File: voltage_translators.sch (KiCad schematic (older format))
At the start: 31 parts, among them IC201 GTL2003PW, IC202 GTL2003PW, IC203 GTL2003PW, IC204 GTL2003PW, IC205 GTL2003PW

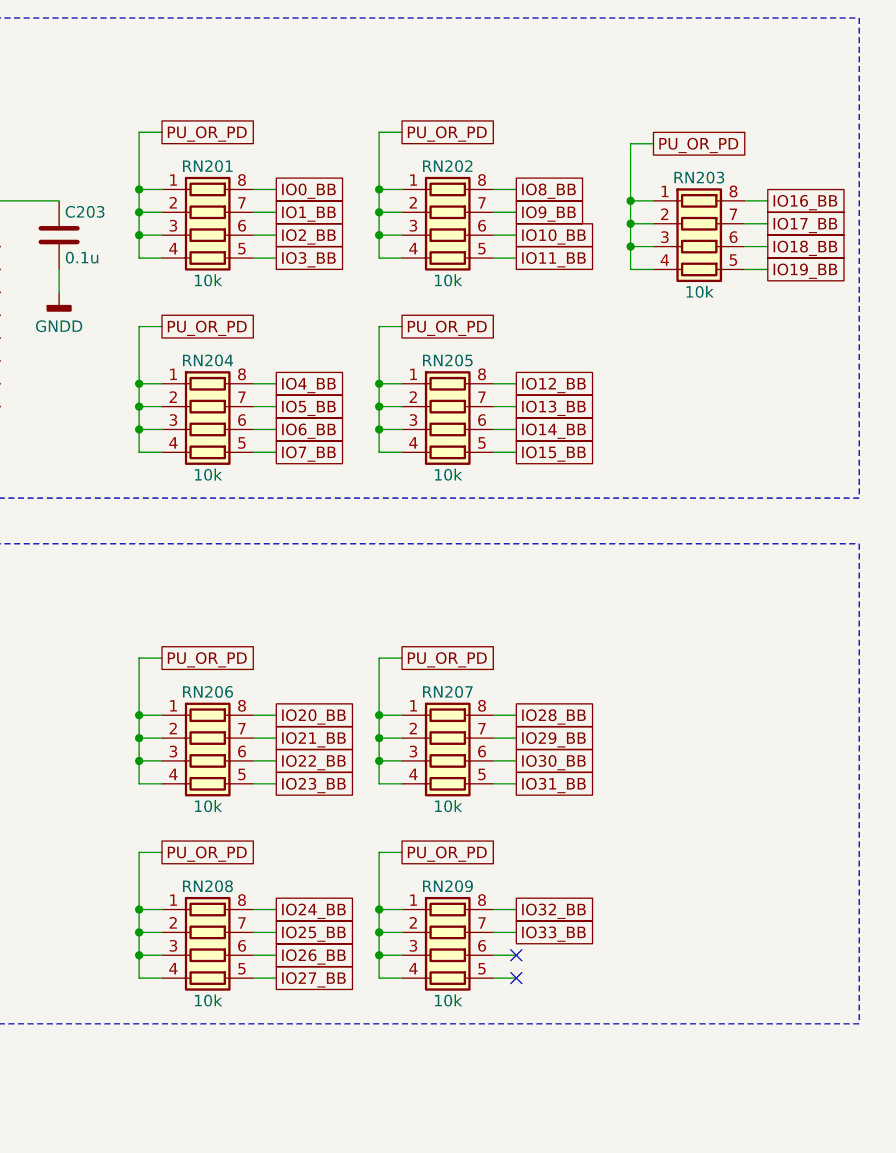
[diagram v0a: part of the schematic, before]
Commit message: revision 1.1 before via stitching
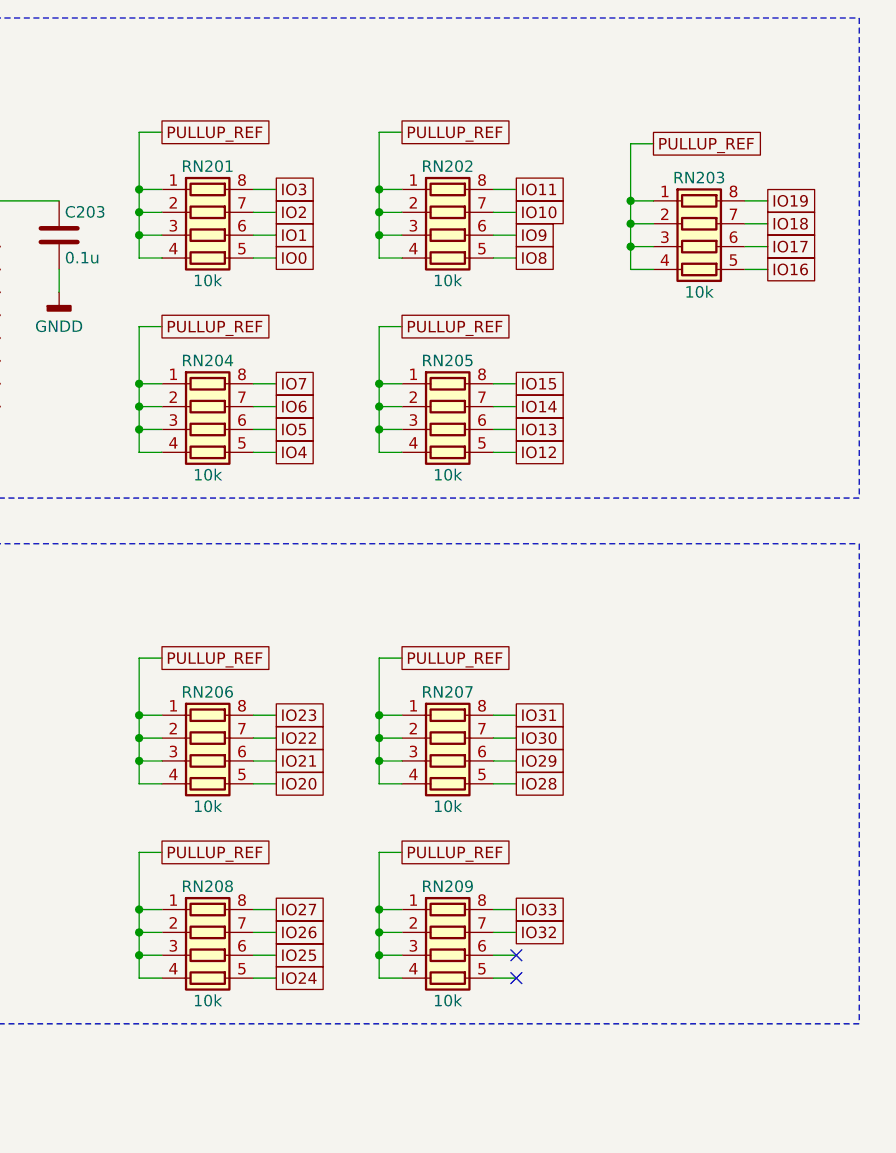
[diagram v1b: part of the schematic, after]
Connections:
- net IO0: now also RN201.5 (R4.2)
- net IO0_BB: no longer RN201.8 (R1.2)
- net IO1: now also RN201.6 (R3.2)
- net IO10: now also RN202.7 (R2.2)
- net IO10_BB: no longer RN202.6 (R3.2)
- net IO11: now also RN202.8 (R1.2)
- net IO11_BB: no longer RN202.5 (R4.2)
- net IO12: now also RN205.5 (R4.2)
- net IO12_BB: no longer RN205.8 (R1.2)
- net IO13: now also RN205.6 (R3.2)
- net IO13_BB: no longer RN205.7 (R2.2)
- net IO14: now also RN205.7 (R2.2)
- net IO14_BB: no longer RN205.6 (R3.2)
- net IO15: now also RN205.8 (R1.2)
- net IO15_BB: no longer RN205.5 (R4.2)
- net IO16: now also RN203.5 (R4.2)
- net IO16_BB: no longer RN203.8 (R1.2)
- net IO17: now also RN203.6 (R3.2)
- net IO17_BB: no longer RN203.7 (R2.2)
- net IO18: now also RN203.7 (R2.2)
- net IO18_BB: no longer RN203.6 (R3.2)
- net IO19: now also RN203.8 (R1.2)
- net IO19_BB: no longer RN203.5 (R4.2)
- net IO1_BB: no longer RN201.7 (R2.2)
- net IO2: now also RN201.7 (R2.2)
- net IO20: now also RN206.5 (R4.2)
- net IO20_BB: no longer RN206.8 (R1.2)
- net IO21: now also RN206.6 (R3.2)
- net IO21_BB: no longer RN206.7 (R2.2)
- net IO22: now also RN206.7 (R2.2)
- net IO22_BB: no longer RN206.6 (R3.2)
- net IO23: now also RN206.8 (R1.2)
- net IO23_BB: no longer RN206.5 (R4.2)
- net IO24: now also RN208.5 (R4.2)
- net IO24_BB: no longer RN208.8 (R1.2)
- net IO25: now also RN208.6 (R3.2)
- net IO25_BB: no longer RN208.7 (R2.2)
- net IO26: now also RN208.7 (R2.2)
- net IO26_BB: no longer RN208.6 (R3.2)
- net IO27: now also RN208.8 (R1.2)
- net IO27_BB: no longer RN208.5 (R4.2)
- net IO28: now also RN207.5 (R4.2)
- net IO28_BB: no longer RN207.8 (R1.2)
- net IO29: now also RN207.6 (R3.2)
- net IO29_BB: no longer RN207.7 (R2.2)
- net IO2_BB: no longer RN201.6 (R3.2)
- net IO3: now also RN201.8 (R1.2)
- net IO30: now also RN207.7 (R2.2)
- net IO30_BB: no longer RN207.6 (R3.2)
- net IO31: now also RN207.8 (R1.2)
- net IO31_BB: no longer RN207.5 (R4.2)
- net IO32: now also RN209.7 (R2.2)
- net IO32_BB: no longer RN209.8 (R1.2)
- net IO33: now also RN209.8 (R1.2)
- net IO33_BB: no longer RN209.7 (R2.2)
- net IO3_BB: no longer RN201.5 (R4.2)
- net IO4: now also RN204.5 (R4.2)
- net IO4_BB: no longer RN204.8 (R1.2)
- net IO5: now also RN204.6 (R3.2)
- net IO5_BB: no longer RN204.7 (R2.2)
- net IO6: now also RN204.7 (R2.2)
- net IO6_BB: no longer RN204.6 (R3.2)
- net IO7: now also RN204.8 (R1.2)
- net IO7_BB: no longer RN204.5 (R4.2)
- net IO8: now also RN202.5 (R4.2)
- net IO8_BB: no longer RN202.8 (R1.2)
- net IO9: now also RN202.6 (R3.2)
- net IO9_BB: no longer RN202.7 (R2.2)
- net PU_OR_PD renamed PULLUP_REF
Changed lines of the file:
@@
 encoding utf-8
 Sheet 2 2
-Title ""
+Title "BeagleBone Parallel Port Cape"
 Date ""
-Rev ""
-Comp ""
+Rev "1.1"
+Comp "Machine Koder"
 Comment1 ""
 Comment2 ""
@@
 	0    1    1    0
 $EndComp
+Text GLabel 8550 1750 2    50   UnSpc ~ 0
+IO0
+Text GLabel 8550 1650 2    50   UnSpc ~ 0
+IO1
+Text GLabel 8550 1550 2    50   UnSpc ~ 0
+IO2
 Text GLabel 8550 1450 2    50   UnSpc ~ 0
-IO0_BB
-Text GLabel 8550 1550 2    50   UnSpc ~ 0
-IO1_BB
-Text GLabel 8550 1650 2    50   UnSpc ~ 0
-IO2_BB
-Text GLabel 8550 1750 2    50   UnSpc ~ 0
-IO3_BB
+IO3
 $Comp
 L R_Pack04 RN204
@@
 	0    1    1    0
 $EndComp
+Text GLabel 8550 2600 2    50   UnSpc ~ 0
+IO4
+Text GLabel 8550 2500 2    50   UnSpc ~ 0
+IO5
+Text GLabel 8550 2400 2    50   UnSpc ~ 0
+IO6
 Text GLabel 8550 2300 2    50   UnSpc ~ 0
-IO4_BB
-Text GLabel 8550 2400 2    50   UnSpc ~ 0
-IO5_BB
-Text GLabel 8550 2500 2    50   UnSpc ~ 0
-IO6_BB
-Text GLabel 8550 2600 2    50   UnSpc ~ 0
-IO7_BB
+IO7
 $Comp
 L R_Pack04 RN202
@@
 	0    1    1    0
 $EndComp
+Text GLabel 9600 1750 2    50   UnSpc ~ 0
+IO8
+Text GLabel 9600 1650 2    50   UnSpc ~ 0
+IO9
+Text GLabel 9600 1550 2    50   UnSpc ~ 0
+IO10
 Text GLabel 9600 1450 2    50   UnSpc ~ 0
-IO8_BB
-Text GLabel 9600 1550 2    50   UnSpc ~ 0
-IO9_BB
-Text GLabel 9600 1650 2    50   UnSpc ~ 0
-IO10_BB
-Text GLabel 9600 1750 2    50   UnSpc ~ 0
-IO11_BB
+IO11
 $Comp
 L R_Pack04 RN205
@@
 	0    1    1    0
 $EndComp
+Text GLabel 9600 2600 2    50   UnSpc ~ 0
+IO12
+Text GLabel 9600 2500 2    50   UnSpc ~ 0
+IO13
+Text GLabel 9600 2400 2    50   UnSpc ~ 0
+IO14
 Text GLabel 9600 2300 2    50   UnSpc ~ 0
-IO12_BB
-Text GLabel 9600 2400 2    50   UnSpc ~ 0
-IO13_BB
-Text GLabel 9600 2500 2    50   UnSpc ~ 0
-IO14_BB
-Text GLabel 9600 2600 2    50   UnSpc ~ 0
-IO15_BB
+IO15
 $Comp
 L R_Pack04 RN203
@@
 	0    1    1    0
 $EndComp
+Text GLabel 10700 1800 2    50   UnSpc ~ 0
+IO16
+Text GLabel 10700 1700 2    50   UnSpc ~ 0
+IO17
+Text GLabel 10700 1600 2    50   UnSpc ~ 0
+IO18
 Text GLabel 10700 1500 2    50   UnSpc ~ 0
-IO16_BB
-Text GLabel 10700 1600 2    50   UnSpc ~ 0
-IO17_BB
-Text GLabel 10700 1700 2    50   UnSpc ~ 0
-IO18_BB
-Text GLabel 10700 1800 2    50   UnSpc ~ 0
-IO19_BB
+IO19
 $Comp
 L R_Pack04 RN206
@@
 	0    1    1    0
 $EndComp
+Text GLabel 8550 4050 2    50   UnSpc ~ 0
+IO20
+Text GLabel 8550 3950 2    50   UnSpc ~ 0
+IO21
+Text GLabel 8550 3850 2    50   UnSpc ~ 0
+IO22
 Text GLabel 8550 3750 2    50   UnSpc ~ 0
-IO20_BB
-Text GLabel 8550 3850 2    50   UnSpc ~ 0
-IO21_BB
-Text GLabel 8550 3950 2    50   UnSpc ~ 0
-IO22_BB
-Text GLabel 8550 4050 2    50   UnSpc ~ 0
-IO23_BB
+IO23
 $Comp
 L R_Pack04 RN208
@@
 	0    1    1    0
 $EndComp
+Text GLabel 8550 4900 2    50   UnSpc ~ 0
+IO24
+Text GLabel 8550 4800 2    50   UnSpc ~ 0
+IO25
+Text GLabel 8550 4700 2    50   UnSpc ~ 0
+IO26
 Text GLabel 8550 4600 2    50   UnSpc ~ 0
-IO24_BB
-Text GLabel 8550 4700 2    50   UnSpc ~ 0
-IO25_BB
-Text GLabel 8550 4800 2    50   UnSpc ~ 0
-IO26_BB
-Text GLabel 8550 4900 2    50   UnSpc ~ 0
-IO27_BB
+IO27
 $Comp
 L R_Pack04 RN207
@@
 	0    1    1    0
 $EndComp
+Text GLabel 9600 4050 2    50   UnSpc ~ 0
+IO28
+Text GLabel 9600 3950 2    50   UnSpc ~ 0
+IO29
+Text GLabel 9600 3850 2    50   UnSpc ~ 0
+IO30
 Text GLabel 9600 3750 2    50   UnSpc ~ 0
-IO28_BB
-Text GLabel 9600 3850 2    50   UnSpc ~ 0
-IO29_BB
-Text GLabel 9600 3950 2    50   UnSpc ~ 0
-IO30_BB
-Text GLabel 9600 4050 2    50   UnSpc ~ 0
-IO31_BB
+IO31
 $Comp
 L R_Pack04 RN209
@@
 	0    1    1    0
 $EndComp
+Text GLabel 9600 4700 2    50   UnSpc ~ 0
+IO32
 Text GLabel 9600 4600 2    50   UnSpc ~ 0
-IO32_BB
-Text GLabel 9600 4700 2    50   UnSpc ~ 0
-IO33_BB
+IO33
 NoConn ~ 9600 4800
 NoConn ~ 9600 4900
 Text GLabel 8050 1200 2    50   UnSpc ~ 0
-PU_OR_PD
-Text GLabel 8050 2050 2    50   UnSpc ~ 0
-PU_OR_PD
-Text GLabel 9100 1200 2    50   UnSpc ~ 0
-PU_OR_PD
-Text GLabel 10200 1250 2    50   UnSpc ~ 0
-PU_OR_PD
-Text GLabel 8050 4350 2    50   UnSpc ~ 0
-PU_OR_PD
-Text GLabel 9100 4350 2    50   UnSpc ~ 0
-PU_OR_PD
-Text GLabel 9100 2050 2    50   UnSpc ~ 0
-PU_OR_PD
-Text GLabel 8050 3500 2    50   UnSpc ~ 0
-PU_OR_PD
-Text GLabel 9100 3500 2    50   UnSpc ~ 0
-PU_OR_PD
+PULLUP_REF
 $Comp
 L GNDD #PWR050
@@
 Text Notes 4600 3150 0    60   ~ 0
 Level Shifters and PU Resistors for Port 2
+Text GLabel 9100 1200 2    50   UnSpc ~ 0
+PULLUP_REF
+Text GLabel 10200 1250 2    50   UnSpc ~ 0
+PULLUP_REF
+Text GLabel 8050 2050 2    50   UnSpc ~ 0
+PULLUP_REF
+Text GLabel 9100 2050 2    50   UnSpc ~ 0
+PULLUP_REF
+Text GLabel 8050 3500 2    50   UnSpc ~ 0
+PULLUP_REF
+Text GLabel 9100 3500 2    50   UnSpc ~ 0
+PULLUP_REF
+Text GLabel 9100 4350 2    50   UnSpc ~ 0
+PULLUP_REF
+Text GLabel 8050 4350 2    50   UnSpc ~ 0
+PULLUP_REF
 $EndSCHEMATC
